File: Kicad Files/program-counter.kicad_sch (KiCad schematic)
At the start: 39 parts, among them U15 74HC245, U16 74HC245, U17 74LS161, U18 74LS161, U19 74LS161, U20 74LS161

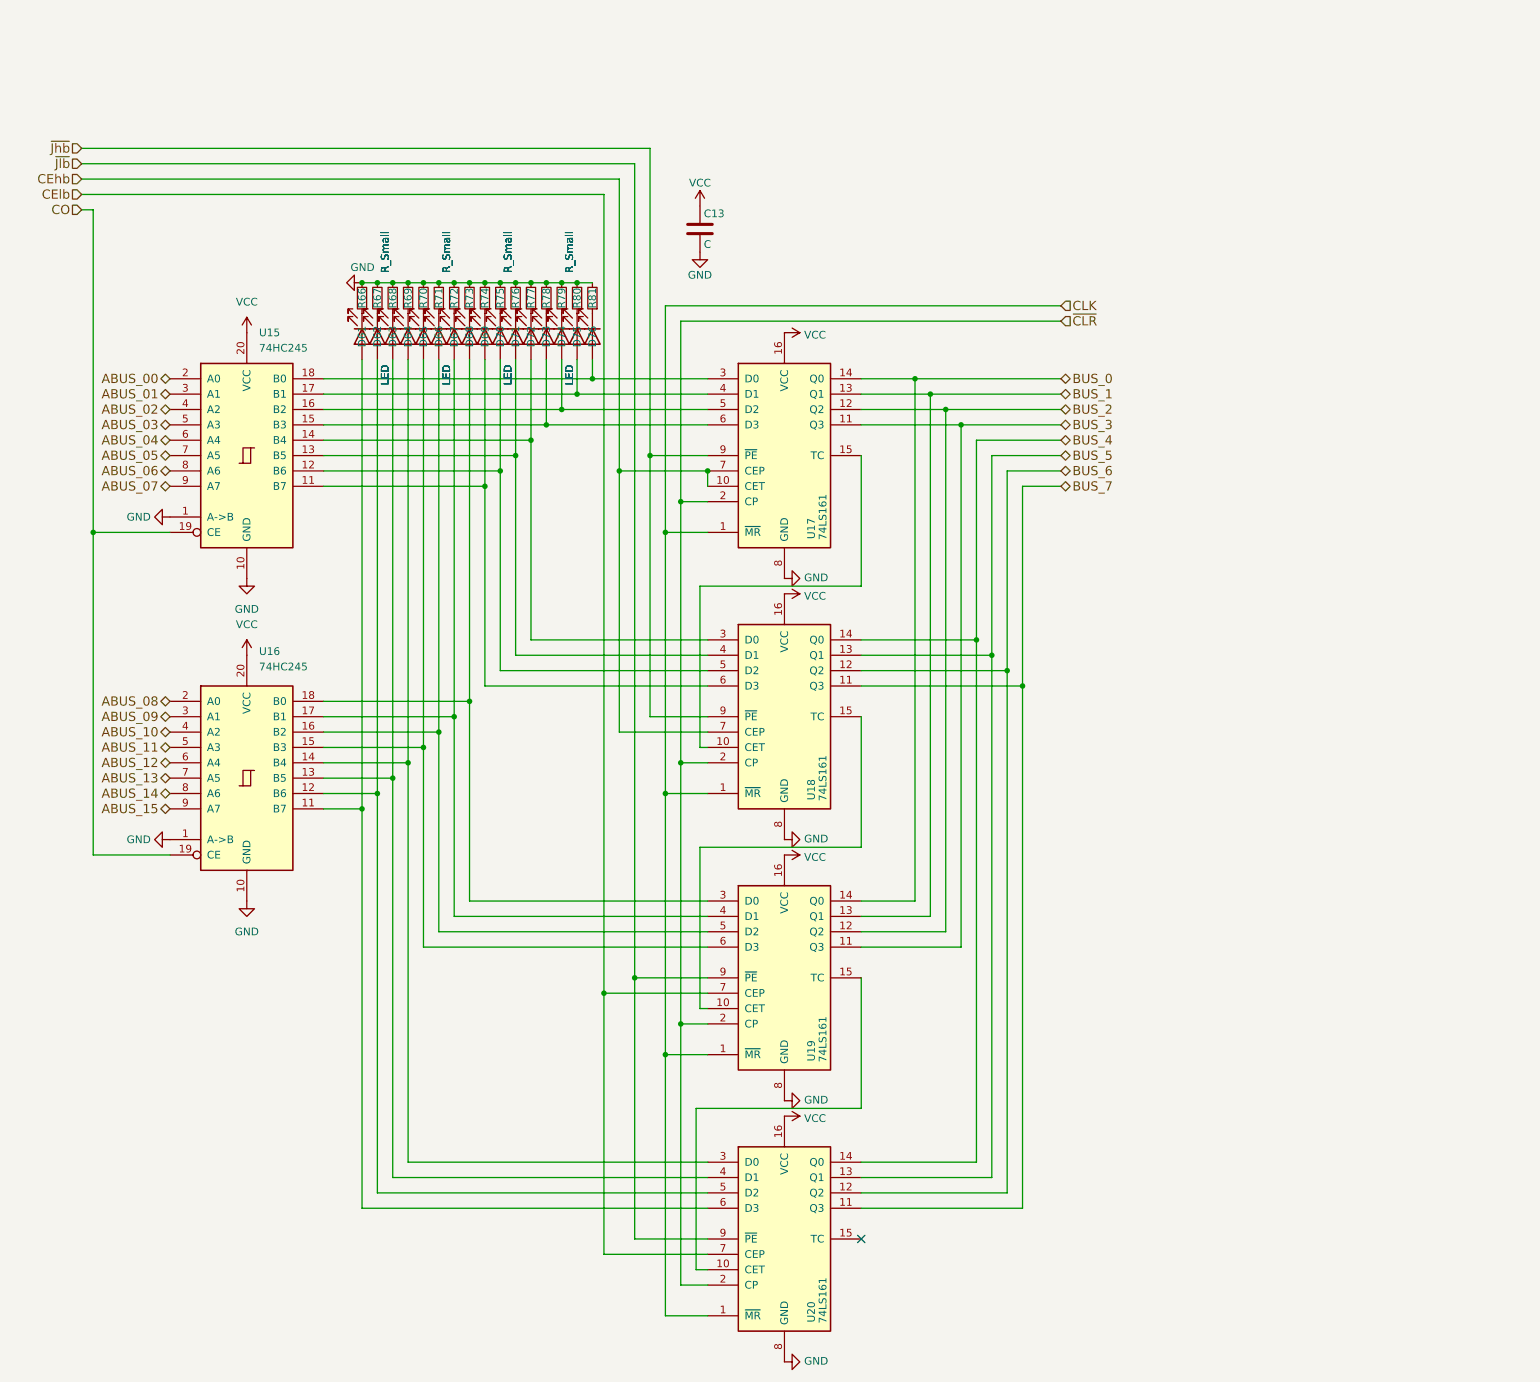
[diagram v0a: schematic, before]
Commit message: np2
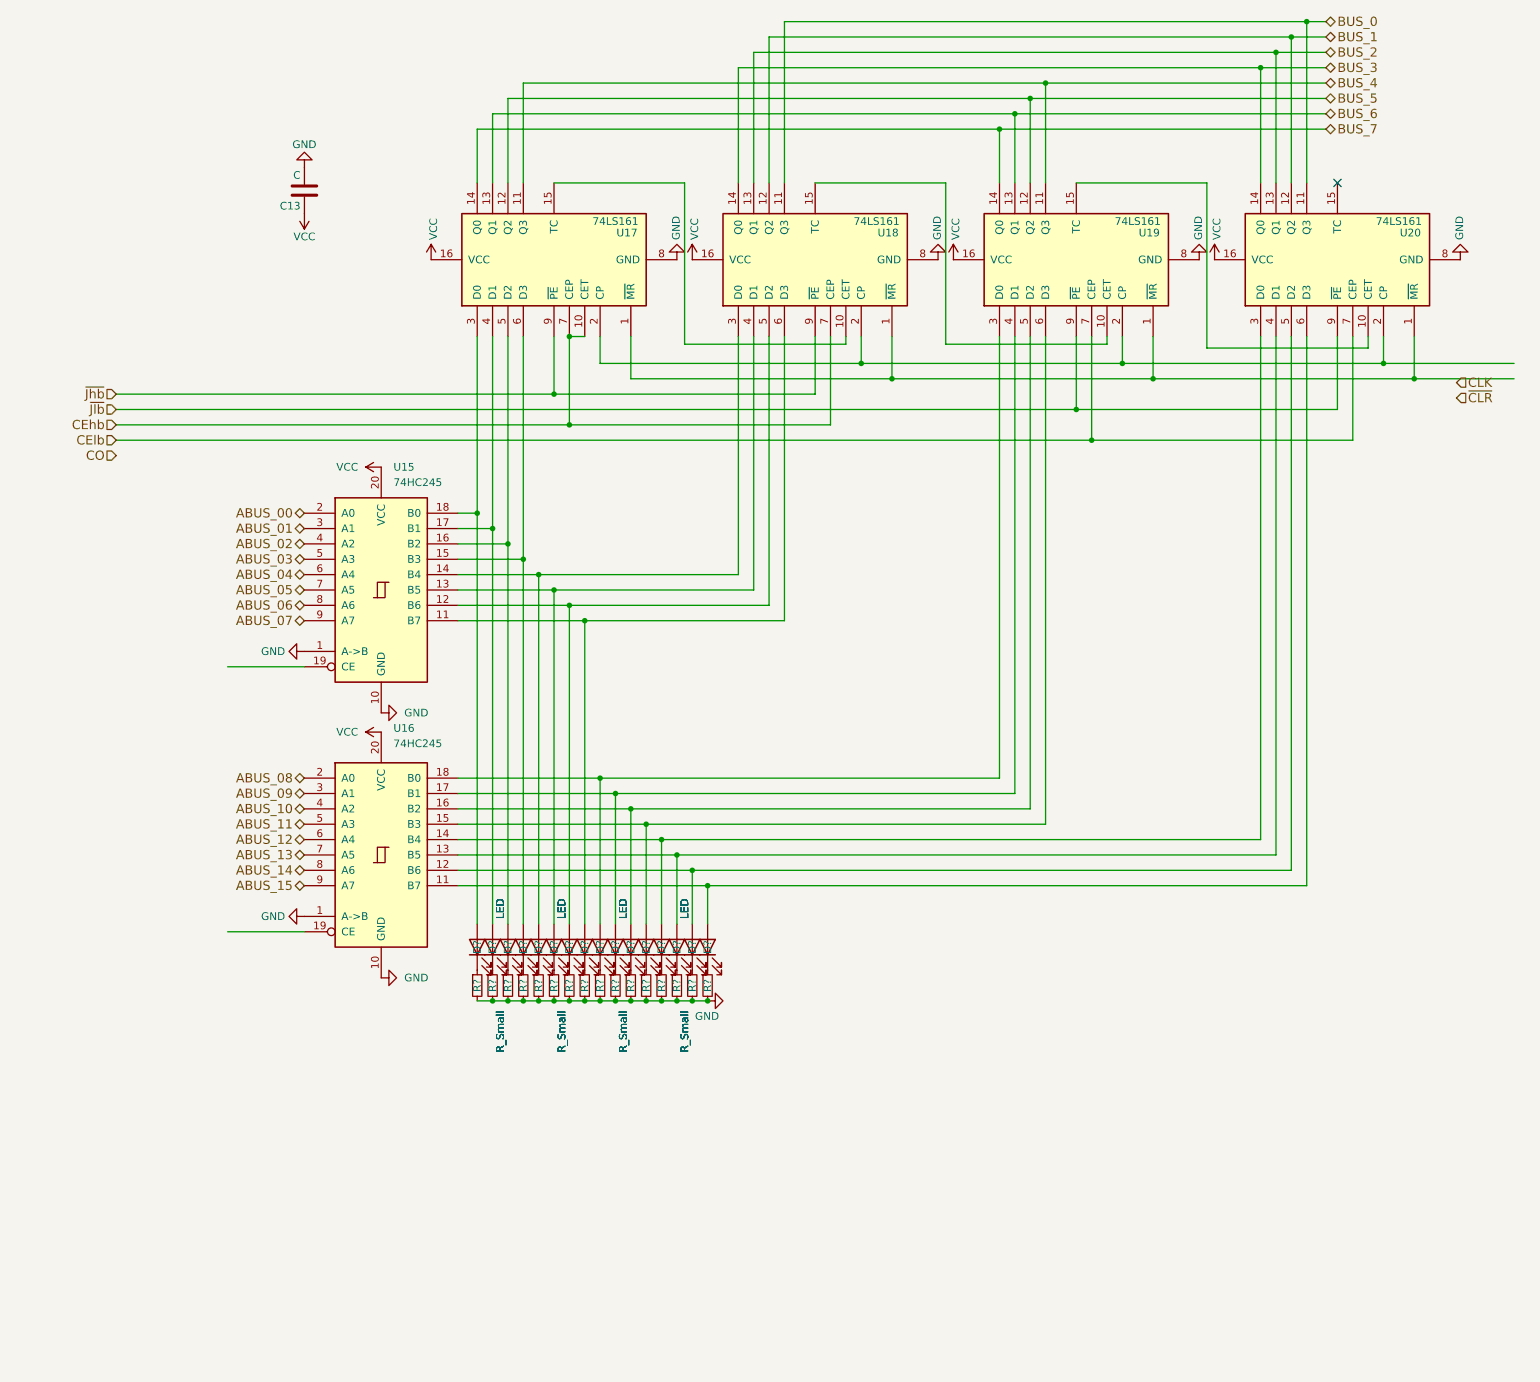
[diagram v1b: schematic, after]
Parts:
- removed D61, D62, D63, D64, D65, D66, D67, D68, D69, D70, D71, D72, D73, D74, D75, D76: LED, symbol Device:LED
- removed R66, R67, R68, R69, R70, R71, R72, R73, R74, R75, R76, R77, R78, R79, R80, R81: R_Small, symbol Device:R_Small
- added D? (x16): LED, symbol Device:LED
- added R? (x16): R_Small, symbol Device:R_Small
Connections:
- net BUS_0: now also U18.11 (Q3), U20.11 (Q3); no longer U17.14 (Q0), U19.14 (Q0)
- net BUS_1: now also U18.12 (Q2), U20.12 (Q2); no longer U17.13 (Q1), U19.13 (Q1)
- net BUS_2: now also U18.13 (Q1), U20.13 (Q1); no longer U17.12 (Q2), U19.12 (Q2)
- net BUS_3: now also U18.14 (Q0), U20.14 (Q0); no longer U17.11 (Q3), U19.11 (Q3)
- net BUS_4: now also U17.11 (Q3), U19.11 (Q3); no longer U18.14 (Q0), U20.14 (Q0)
- net BUS_5: now also U17.12 (Q2), U19.12 (Q2); no longer U18.13 (Q1), U20.13 (Q1)
- net BUS_6: now also U17.13 (Q1), U19.13 (Q1); no longer U18.12 (Q2), U20.12 (Q2)
- net BUS_7: now also U17.14 (Q0), U19.14 (Q0); no longer U18.11 (Q3), U20.11 (Q3)
- net CLK: no longer U17.1 (~{MR}), U18.1 (~{MR}), U19.1 (~{MR}), U20.1 (~{MR})
- net CO: no longer U15.19 (CE), U16.19 (CE)
- net GND: now also R?.2, R?.2, R?.2, R?.2, R?.2, R?.2, R?.2, R?.2, R?.2, R?.2, R?.2, R?.2, R?.2, R?.2, R?.2, R?.2
- net ~{CLR}: no longer U17.2 (CP), U18.2 (CP), U19.2 (CP), U20.2 (CP)
- net at U15.15 (B3), U17.6 (D3): now also D?.2 (A)
- net at U16.12 (B6), U20.5 (D2): now also D?.2 (A)
- net at U15.18 (B0), U17.3 (D0): now also D?.2 (A)
- net at U16.11 (B7), U20.6 (D3): now also D?.2 (A)
- net at U16.13 (B5), U20.4 (D1): now also D?.2 (A)
- net at U16.14 (B4), U20.3 (D0): now also D?.2 (A)
- net at U16.15 (B3), U19.6 (D3): now also D?.2 (A)
- net at U16.16 (B2), U19.5 (D2): now also D?.2 (A)
- net at U16.17 (B1), U19.4 (D1): now also D?.2 (A)
- net at U16.18 (B0), U19.3 (D0): now also D?.2 (A)
- net at U15.12 (B6), U18.5 (D2): now also D?.2 (A)
- net at U15.17 (B1), U17.4 (D1): now also D?.2 (A)
- net at U15.14 (B4), U18.3 (D0): now also D?.2 (A)
- net at U15.13 (B5), U18.4 (D1): now also D?.2 (A)
- net at U15.11 (B7), U18.6 (D3): now also D?.2 (A)
- net at U15.16 (B2), U17.5 (D2): now also D?.2 (A)
- new net: D?.1 (K), R?.1 (x16)
- new net: U17.1 (~{MR}), U18.1 (~{MR}), U19.1 (~{MR}), U20.1 (~{MR})
- new net: U17.2 (CP), U18.2 (CP), U19.2 (CP), U20.2 (CP)
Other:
- moved on the sheet: C13, U15, U16, U17, U18, U19, U20
